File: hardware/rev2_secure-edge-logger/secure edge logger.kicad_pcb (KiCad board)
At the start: 4 copper layers, 87.5 x 54.7 mm, 105 parts, among them IC1 BQ27441DRZT-G1A, IC2 TPS63802DLAR, J1 SS-52400-002, J2 B2B-PH-SM4-TB, J3 GSD090012SEU, Q1 TEMT6000X01, Q2 BC817, Q3 BC817, U1 MCP73871-2CAI_ML, U2 CP2102N-Axx-xQFN20, U3 ESP32-C3-WROOM-02-H4, U4 W25Q32JVSSIQ, U5 USBLC6-2SC6, U6 BME280, U7 MAX4466EXK, U8 ds3231sn-, U9 SE050E2HQ1/Z01Z3Z

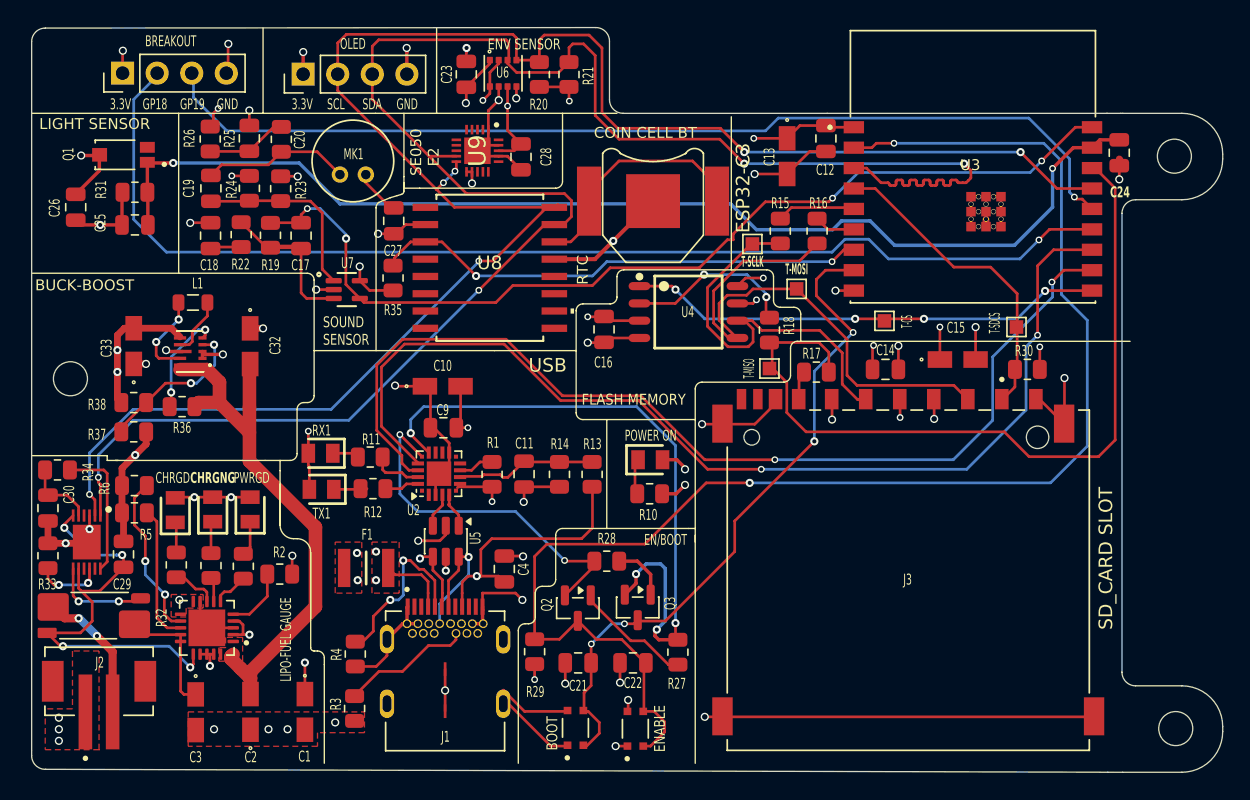
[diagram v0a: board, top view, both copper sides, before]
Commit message: Add files via upload
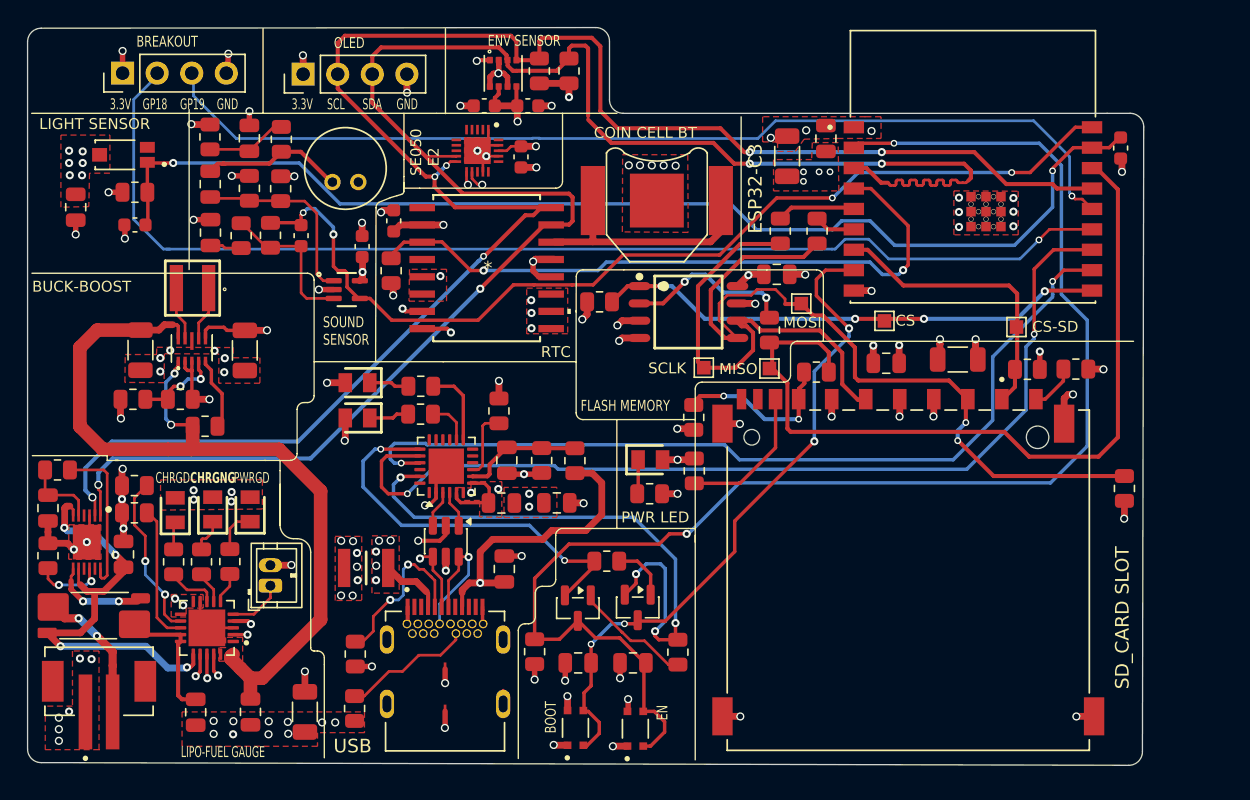
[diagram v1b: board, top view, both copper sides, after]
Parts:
- removed J1: SS-52400-002, ESP32Footprints:BELFUSE_SS-52400-002
- removed L1: 0.47uH, Inductor_SMD:L_0805_2012Metric
- removed MH01 (x3): MountingHole_2.5mm, MountingHole:MountingHole_2.5mm
- removed R2: 10K, Resistor_SMD:R_0805_2012Metric
- removed U2: CP2102N-Axx-xQFN20, Package_DFN_QFN:SiliconLabs_QFN-20-1EP_3x3mm_P0.5mm_EP1.8x1.8mm
- removed U8: ds3231sn-, ESP32Footprints:21-0042B_16_MXM
- removed U9: SE050E2HQ1/Z01Z3Z, ESP32Footprints:QFN40P300X300X33-21N-D
- added C310: 100n, Capacitor_SMD:C_0603_1608Metric, F.Cu at (189.2, 81.5)
- added C311: 100n, Capacitor_SMD:C_0603_1608Metric, F.Cu at (180.3, 91.8)
- added J100: SS-52400-003, ESP32Footprints:BELFUSE_SS-52400-003, F.Cu at (186.4, 125.4)
- added J102: Conn_01x02, Connector_JST:JST_ZH_B2B-ZR_1x02_P1.50mm_Vertical, F.Cu at (173.5, 116.7)
- added L100: XFL4015-471MEC, ESP32Footprints:XFL4012, F.Cu at (167.8, 94.8)
- added R210: 10k, Resistor_SMD:R_0805_2012Metric, F.Cu at (236.3, 109.6)
- added R211: 10k, Resistor_SMD:R_0805_2012Metric, F.Cu at (204.6, 104.3)
- added R212: 10k, Resistor_SMD:R_0805_2012Metric, F.Cu at (204.7, 108.3)
- added R213: 10k, Resistor_SMD:R_0805_2012Metric, F.Cu at (232.7, 100.8)
- added R214: 10k, Resistor_SMD:R_0805_2012Metric, F.Cu at (197.7, 95.8)
- added U200: CP2102N-Axx-xQFN24, Package_DFN_QFN:QFN-24-1EP_4x4mm_P0.5mm_EP2.6x2.6mm, F.Cu at (186.5, 107.9)
- added U301: ds3231sn-, ESP32Footprints:21-0042B_16_MXM, F.Cu at (189.4, 93.4)
- added U302: SE050E2HQ1/Z01Z3Z, ESP32Footprints:QFN40P300X300X33-21N-D, F.Cu at (188.8, 84.8)
- BT300: renamed from BT1; value CR2032 -> Keystone 2998
- C101: renamed from C1; footprint ESP32Footprints:T491A -> Capacitor_SMD:C_1206_3216Metric
- C102: renamed from C2; footprint ESP32Footprints:T491A -> Capacitor_SMD:C_0805_2012Metric
- C103: renamed from C32; footprint ESP32Footprints:T491A -> Capacitor_SMD:C_1206_3216Metric
- C104: renamed from C33; footprint ESP32Footprints:T491A -> Capacitor_SMD:C_1206_3216Metric
- C107: renamed from C3; footprint ESP32Footprints:T491A -> Capacitor_SMD:C_0805_2012Metric
- C200: renamed from C10; footprint ESP32Footprints:T491A -> Capacitor_SMD:C_0805_2012Metric
- C204: renamed from C12; value 0.1U -> 0.1u
- C205: renamed from C13; value 1Ou -> 10u; footprint ESP32Footprints:T491A -> Capacitor_SMD:C_1206_3216Metric
- C206: renamed from C15; footprint ESP32Footprints:T491A -> Capacitor_SMD:C_1206_3216Metric
- C300: renamed from C23; footprint Capacitor_SMD:C_0805_2012Metric -> Capacitor_SMD:C_0603_1608Metric
- C301: renamed from C24; footprint Capacitor_SMD:C_0805_2012Metric -> Capacitor_SMD:C_0603_1608Metric
- C302: renamed from C25; footprint Capacitor_SMD:C_0805_2012Metric -> Capacitor_SMD:C_0603_1608Metric
- C303: renamed from C27; footprint Capacitor_SMD:C_0805_2012Metric -> Capacitor_SMD:C_0603_1608Metric
- C304: renamed from C28; footprint Capacitor_SMD:C_0805_2012Metric -> Capacitor_SMD:C_0603_1608Metric
- C308: renamed from C17; footprint Capacitor_SMD:C_0805_2012Metric -> Capacitor_SMD:C_0603_1608Metric
- C400: renamed from C21; value 0.1u -> DNP
- C401: renamed from C22; value 0.1u -> 1u
- PWR100: renamed from POWER ON
- U203: renamed from U3; footprint ESP32Footprints:MODULE_ESP32-C3-WROOM-02-H4 -> ESP32Footprints:ESP32--C3-WROOM-02-H4
- moved C203 13.3 mm to (210.7, 93.8), turned to 180 degrees
- moved C200 12.0 mm to (194.6, 110.6), turned to 180 degrees
- moved TP5 9.77 mm to (205.4, 100.7)
- moved C104 8.17 mm to (171.7, 99.4)
- moved C103 8.07 mm to (164.0, 99.4), turned to 90 degrees
- moved C201 6.98 mm to (190.5, 110.6), turned to 180 degrees
- moved R203 6.50 mm to (184.6, 104.1)
- moved R204 6.39 mm to (184.6, 102.0)
- moved TX200 5.87 mm to (179.9, 104.4)
- moved RX200 5.85 mm to (179.9, 101.8)
- moved C300 5.08 mm to (192.4, 81.5), turned to 0 degrees
- moved R200 4.69 mm to (190.3, 103.9), turned to -90 degrees
- moved R109 4.17 mm to (166.9, 103.0)
- moved R110 2.22 mm to (168.7, 105.0), turned to 180 degrees
- moved R202 1.65 mm to (193.5, 107.5)
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- renumbered BREAKOUT to BREAKOUT400, C4 to C100, C30 to C105, C29 to C106, C9 to C201, C11 to C202, C16 to C203, C14 to C207, C20 to C305, C19 to C306, C18 to C307, C26 to C309, LED1 to D100, LED3 to D101, LED2 to D102, F1 to F100, IC2 to IC100, IC1 to IC101, J2 to J101, J3 to J200, MK1 to MK300, OLED to OLED400, Q1 to Q300, Q2 to Q400, Q3 to Q401, R4 to R100, R3 to R101, R7 to R102, R8 to R103, R9 to R104, R32 to R105, R6 to R107, R38 to R108, R37 to R109, R36 to R110, R10 to R111, R34 to R112, R33 to R113, R5 to R114, R1 to R200, R13 to R201, R14 to R202, R12 to R203, R11 to R204, R18 to R205, R15 to R206, R16 to R207, R17 to R208, R30 to R209, R21 to R300, R20 to R301, R31 to R302, R35 to R303, R26 to R304, R25 to R305, R24 to R306, R22 to R307, R23 to R308, R19 to R309, R27 to R400, R28 to R401, R29 to R402, RX1 to RX200, BOOT to S400, ENABLE to S401, T-MISO to TP1, T-MOSI to TP2, T-SDCS to TP3, T-CS to TP4, T-SCLK to TP5, TX1 to TX200, U1 to U100, U5 to U201, U4 to U202, U6 to U300, U7 to U303
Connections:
- net /ESP32-C3-02/DTS renamed /ESP32-C3-02/DTR
- net Net-(J3-DAT0) renamed /ESP32-C3-02/MISO-GSD
- net Net-(U2-VBUS) renamed /ESP32-C3-02/VBUS-CP
- net Net-(U3-IO6) renamed /ESP32-C3-02/SCLK-ESP
- net Net-(U3-IO7) renamed /ESP32-C3-02/MISO-ESP
- net Net-(U4-DO(IO1)) renamed /ESP32-C3-02/MISO-W25
- BT300 pad 1: Net-(BT1-+) -> /ESP32-C3-02/SENSORS/VBAT-DS
- C200 pad 1: GND -> +3.3V
- C200 pad 2: +3.3V -> GND
- J200 pad 8: GND -> /ESP32-C3-02/DAT1
- J200 pad 9: GND -> /ESP32-C3-02/DAT2
- R200 pad 2: Net-(U2-~{RST}) -> /ESP32-C3-02/NRST
- R203 pad 1: Net-(U2-~{TXT}/GPIO.2) -> /ESP32-C3-02/NTXT
- R204 pad 1: Net-(U2-~{RXT}/GPIO.3) -> /ESP32-C3-02/NRXT
- U100 pad 5: Net-(U1-THERM) -> /THERM
- U203 pad 4: /ESP32-C3-02/CS-SD -> /ESP32-C3-02/INT/SQW
- U203 pad 7: /ESP32-C3-02/INT/SQW -> /ESP32-C3-02/CS-SD
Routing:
- net GND: track 193.1 -> 100.5 mm, vias 49 -> 97
- net /MCP-OUT: track 41.2 -> 62.9 mm, vias 0 -> 2
- net /ESP32-C3-02/SENSORS/VBAT-DS: track 0.00 -> 18.9 mm
- net +3.3V: track 82.0 -> 64.0 mm, vias 27 -> 44
- net Net-(BT1-+): track 17.7 -> 0.00 mm
- net /ESP32-C3-02/MOSI-DI: track 40.4 -> 57.5 mm, vias 0 -> 2
- net /ESP32-C3-02/INT/SQW: track 36.7 -> 48.3 mm
- net /ESP32-C3-02/DAT1: track 0.00 -> 11.5 mm
- net /ESP32-C3-02/TX-RX: track 75.8 -> 64.5 mm
- net /ESP32-C3-02/MISO-GSD: track 2.18 -> 12.5 mm, vias 0 -> 2
- net /ESP32-C3-02/DTR: track 49.9 -> 43.2 mm
- net /ESP32-C3-02/RX-TX: track 77.3 -> 70.6 mm
- net /ESP32-C3-02/NRXT: track 0.00 -> 5.74 mm
- net Net-(IC100-FB): track 11.5 -> 6.38 mm
- net /ESP32-C3-02/NRST: track 0.00 -> 5.04 mm
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- added copper zone on F.Cu, net +3.3V
- added copper zone on In2.Cu, net +3.3V
- added copper zone on In2.Cu, net /+5V-USB
- added copper zone on In2.Cu, net /VBUS
- added copper zone on In1.Cu, net GND
- removed copper zone on In1.Cu, net +3.3V
- removed copper zone on In1.Cu, net /+5V-USB
- removed copper zone on In1.Cu, net /VBUS
- removed copper zone on In2.Cu, net GND
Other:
- board size 87.5 x 54.7 mm -> 82 x 54.2 mm
- board text added: "BOOT"
- board text added: "BREAKOUT"
- board text added: "CS"
- board text added: "CS-SD"
- board text added: "EN"
- board text added: "MISO"
- board text added: "MOSI"
- board text added: "OLED"
- board text added: "PWR LED"
- board text added: "SCLK"
- board text removed: "EN/BOOT"
